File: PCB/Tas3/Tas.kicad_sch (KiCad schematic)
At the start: 27 parts, among them J1 Shelly 1, J2 Conn_01x07, J3 USB-C, U1 MD8942, U2 Barcode, U3 CH340X, U4 ISL89410

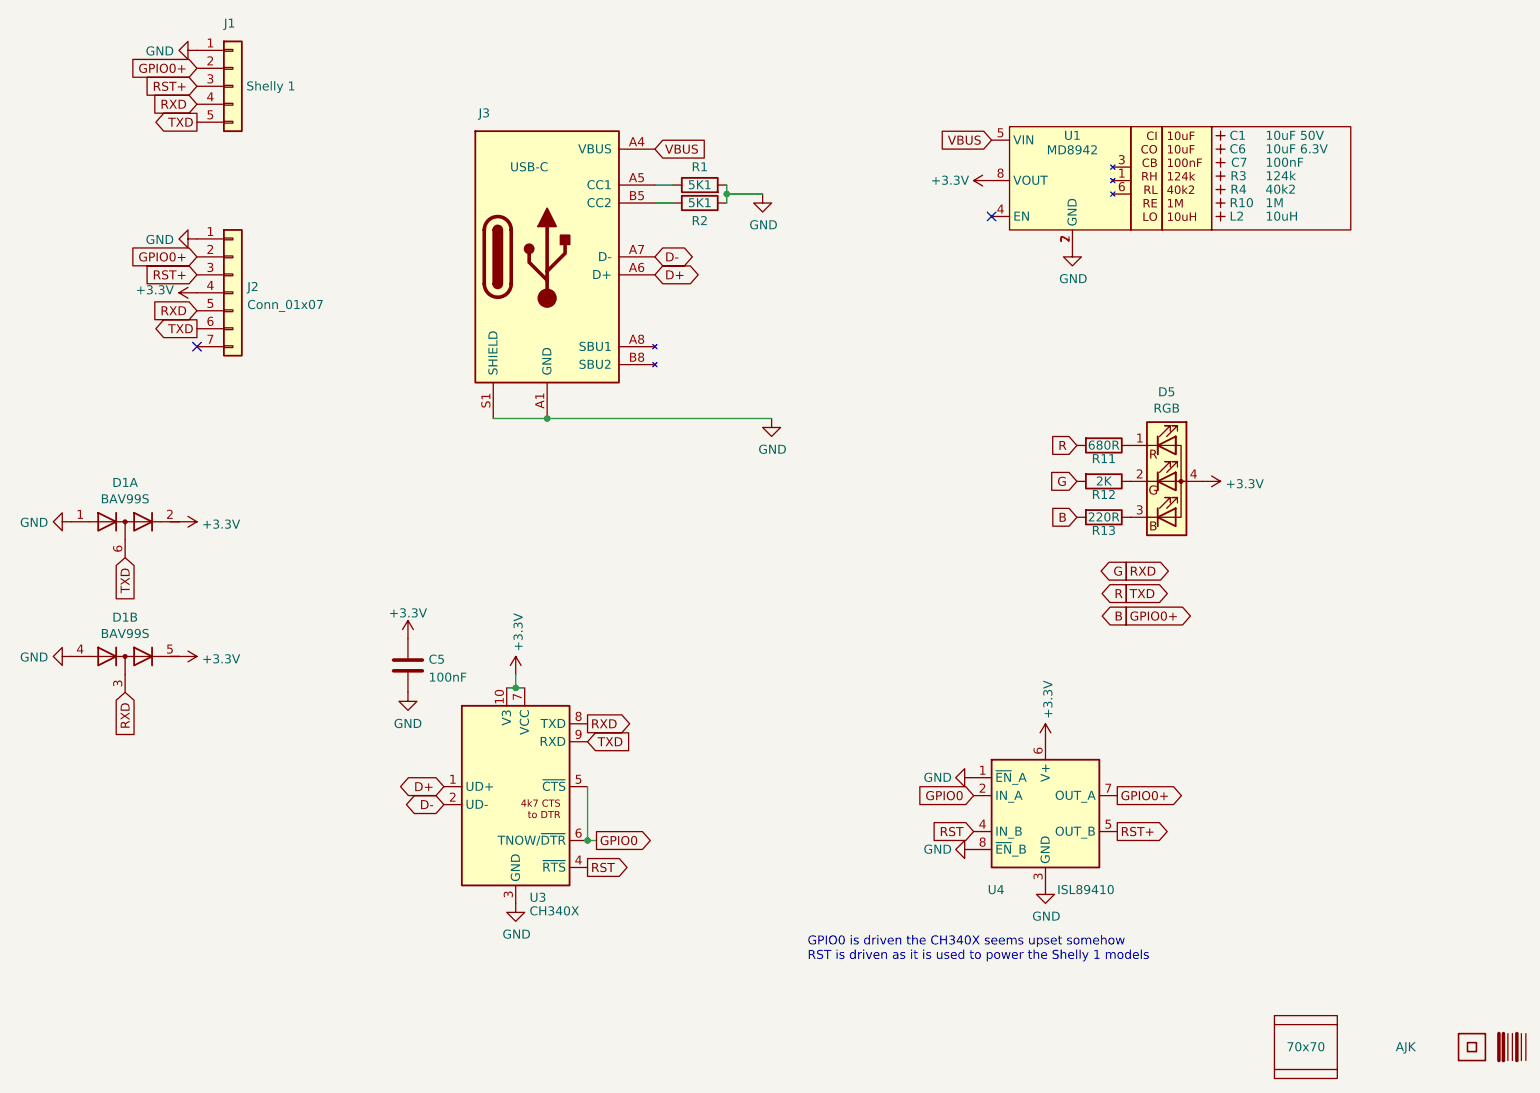
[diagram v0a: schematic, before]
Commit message: As ordered
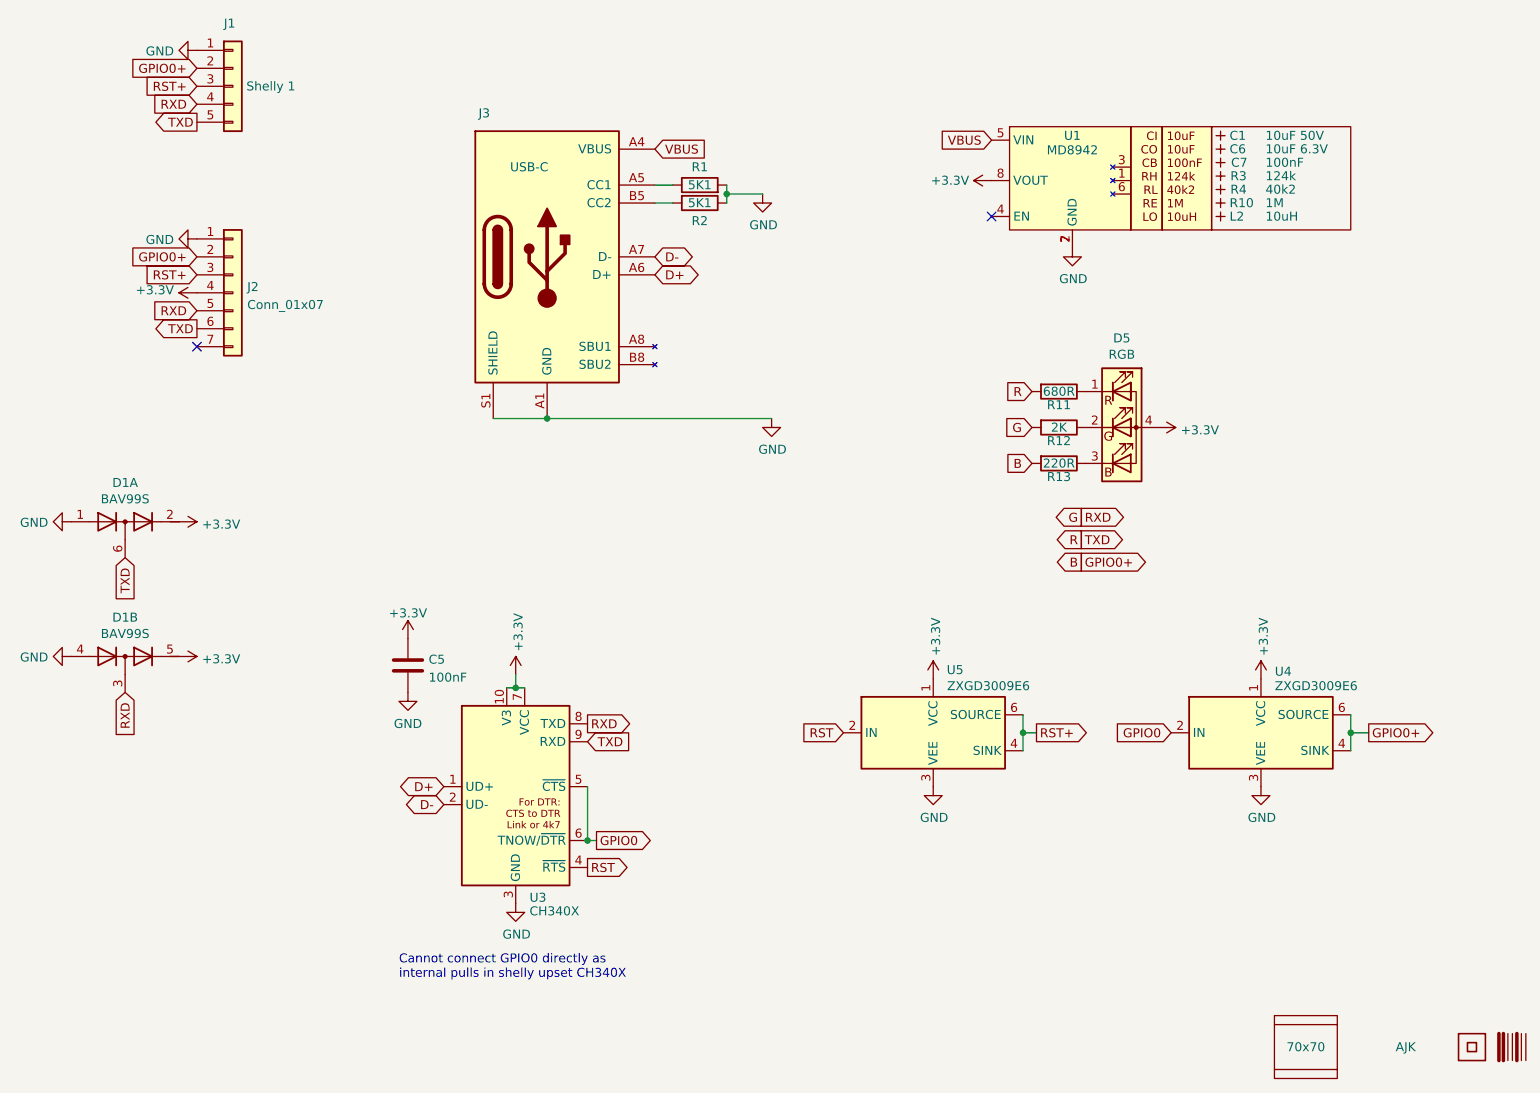
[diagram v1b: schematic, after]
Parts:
- removed U4: ISL89410, RevK:SO-8_3.9x4.9mm_P1.27mm, symbol RevK:IVCR2404
- added U4, U5: ZXGD3009E6, RevK:SOT-23-6, symbol Driver_FET:ZXGD3009E6
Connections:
- net +3V3: now also U4.1 (VCC), U5.1 (VCC)
- net B: now also U4.4 (SINK), U4.6 (SOURCE)
- net GND: now also U4.3 (VEE), U5.3 (VEE)
- net GPIO0: now also U4.2 (IN)
- net RST: now also U5.2 (IN)
- net RST+: now also U5.4 (SINK), U5.6 (SOURCE)
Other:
- note added: "Cannot connect GPIO0 directly as internal pulls in shelly upset CH340X"
- note removed: "GPIO0 is driven the CH340X seems upset somehow RST is driven as it is used to power the Shelly 1 models"
- moved on the sheet: D5, R11, R12, R13
